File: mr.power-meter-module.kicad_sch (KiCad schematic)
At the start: 3 parts

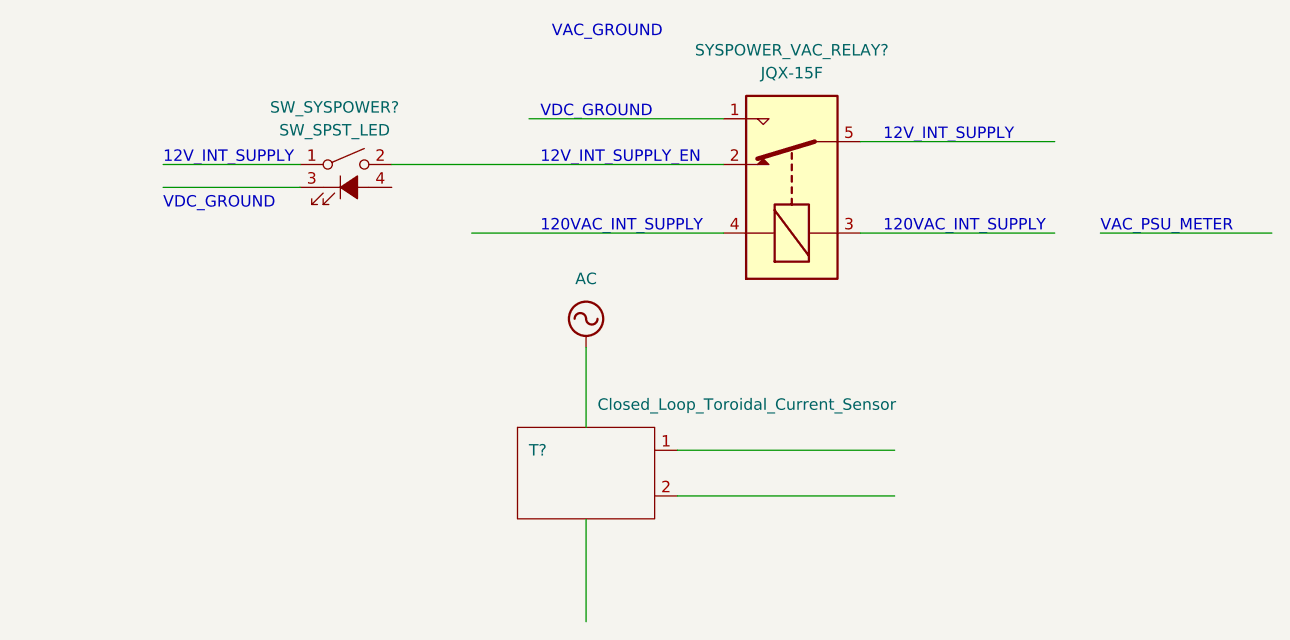
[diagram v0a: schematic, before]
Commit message: Place Holder:
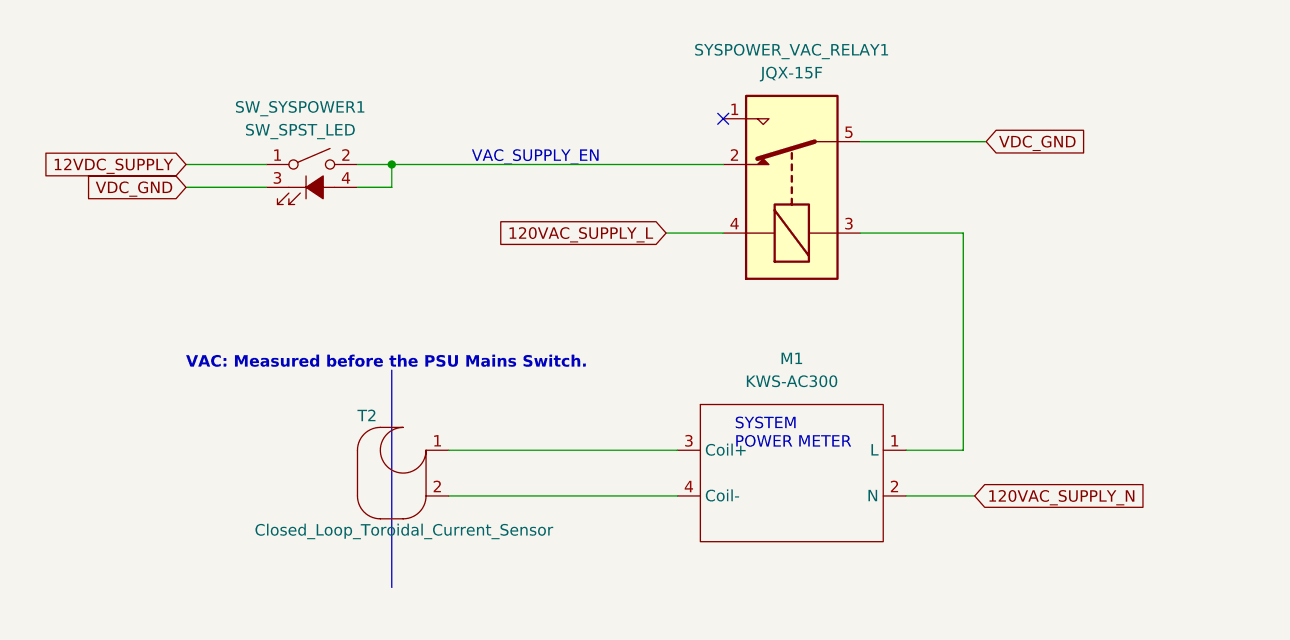
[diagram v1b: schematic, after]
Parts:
- added M1: KWS-AC300, symbol bvm-library:4_Pin_Meter_With_Toroid
- gave numbers to parts that had none: 3
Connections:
- net at SW_SYSPOWER1.2, SYSPOWER_VAC_RELAY1.2: now also SW_SYSPOWER1.4 (A)
- net at SYSPOWER_VAC_RELAY1.3: now also M1.1 (L)
- net 120VAC_SUPPLY_L: now reaches SYSPOWER_VAC_RELAY1.4
- net VDC_GND: now reaches SYSPOWER_VAC_RELAY1.5, SYSPOWER_VAC_RELAY1.6
- net VDC_GND: now also SW_SYSPOWER1.3 (K)
- net at T2.1 (Current_Sense_A): now also M1.3 (Coil+)
- net at T2.2 (Current_Sense_B): now also M1.4 (Coil-)
- net 12VDC_SUPPLY: now reaches SW_SYSPOWER1.1
- new net 120VAC_SUPPLY_N: M1.2 (N)
- no-connect marks 0 -> 1
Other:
- note added: "SYSTEM POWER METER"
- note added: "VAC: Measured before the PSU Mains Switch."
- note added: "VAC_SUPPLY_EN"
- note removed: "120VAC_INT_SUPPLY"
- note removed: "12V_INT_SUPPLY"
- note removed: "12V_INT_SUPPLY_EN"
- note removed: "VAC_GROUND"
- note removed: "VAC_PSU_METER"
- note removed: "VDC_GROUND"
- moved on the sheet: SW_SYSPOWER1
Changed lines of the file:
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@@
     (company "eatmellc")
   )
-  (wire (pts (xy 124.46 63.5) (xy 146.05 63.5))
-    (stroke (width 0) (type default) (color 0 0 0 0))
+  (junction (at 109.22 68.58) (diameter 0) (color 0 0 0 0)
   )
-  (wire (pts (xy 83.82 68.58) (xy 99.06 68.58))
-    (stroke (width 0) (type default) (color 0 0 0 0))
-  )
-  (wire (pts (xy 140.97 100.33) (xy 165.1 100.33))
-    (stroke (width 0) (type default) (color 0 0 0 0))
-  )
-  (wire (pts (xy 187.96 76.2) (xy 207.01 76.2))
-    (stroke (width 0) (type default) (color 0 0 0 0))
-  )
-  (wire (pts (xy 118.11 76.2) (xy 146.05 76.2))
-    (stroke (width 0) (type default) (color 0 0 0 0))
-  )
-  (wire (pts (xy 130.81 107.95) (xy 130.81 119.38))
-    (stroke (width 0) (type default) (color 0 0 0 0))
-  )
-  (wire (pts (xy 83.82 71.12) (xy 99.06 71.12))
+  (no_connect (at 146.05 63.5))
+  (wire (pts (xy 109.22 68.58) (xy 109.22 71.12))
     (stroke (width 0) (type default) (color 0 0 0 0))
   )
@@
     (stroke (width 0) (type default) (color 0 0 0 0))
   )
-  (wire (pts (xy 161.29 66.04) (xy 182.88 66.04))
+  (wire (pts (xy 86.36 68.58) (xy 95.25 68.58))
     (stroke (width 0) (type default) (color 0 0 0 0))
   )
-  (wire (pts (xy 161.29 76.2) (xy 182.88 76.2))
+  (wire (pts (xy 172.72 100.33) (xy 172.72 76.2))
     (stroke (width 0) (type default) (color 0 0 0 0))
   )
-  (wire (pts (xy 140.97 105.41) (xy 165.1 105.41))
+  (wire (pts (xy 109.22 71.12) (xy 105.41 71.12))
     (stroke (width 0) (type default) (color 0 0 0 0))
   )
-  (wire (pts (xy 130.81 88.9) (xy 130.81 97.79))
+  (wire (pts (xy 139.7 76.2) (xy 146.05 76.2))
     (stroke (width 0) (type default) (color 0 0 0 0))
   )
-  (text "12V_INT_SUPPLY" (at 163.83 66.04 0)
+  (wire (pts (xy 166.37 100.33) (xy 172.72 100.33))
+    (stroke (width 0) (type default) (color 0 0 0 0))
+  )
+  (wire (pts (xy 105.41 68.58) (xy 109.22 68.58))
+    (stroke (width 0) (type default) (color 0 0 0 0))
+  )
+  (wire (pts (xy 115.57 100.33) (xy 140.97 100.33))
+    (stroke (width 0) (type default) (color 0 0 0 0))
+  )
+  (wire (pts (xy 161.29 66.04) (xy 175.26 66.04))
+    (stroke (width 0) (type default) (color 0 0 0 0))
+  )
+  (wire (pts (xy 161.29 76.2) (xy 172.72 76.2))
+    (stroke (width 0) (type default) (color 0 0 0 0))
+  )
+  (wire (pts (xy 115.57 105.41) (xy 140.97 105.41))
+    (stroke (width 0) (type default) (color 0 0 0 0))
+  )
+  (polyline (pts (xy 109.22 91.44) (xy 109.22 115.57))
+    (stroke (width 0) (type default) (color 0 0 0 0))
+  )
+  (wire (pts (xy 166.37 105.41) (xy 173.99 105.41))
+    (stroke (width 0) (type default) (color 0 0 0 0))
+  )
+  (wire (pts (xy 86.36 71.12) (xy 95.25 71.12))
+    (stroke (width 0) (type default) (color 0 0 0 0))
+  )
+  (text "VAC_SUPPLY_EN" (at 118.11 68.58 0)
     (effects (font (size 1.27 1.27)) (justify left bottom))
   )
-  (text "VAC_GROUND" (at 127 54.61 0)
+  (text "SYSTEM\nPOWER METER" (at 147.32 100.33 0)
     (effects (font (size 1.27 1.27)) (justify left bottom))
   )
-  (text "VDC_GROUND" (at 83.82 73.66 0)
-    (effects (font (size 1.27 1.27)) (justify left bottom))
+  (text "VAC: Measured before the PSU Mains Switch." (at 86.36 91.44 0)
+    (effects (font (size 1.27 1.27) (thickness 0.254) bold) (justify left bottom))
   )
-  (text "12V_INT_SUPPLY_EN" (at 125.73 68.58 0)
-    (effects (font (size 1.27 1.27)) (justify left bottom))
+  (global_label "120VAC_SUPPLY_L" (shape input) (at 139.7 76.2 180) (fields_autoplaced)
+    (effects (font (size 1.27 1.27)) (justify right))
+    (property "Intersheet References" "${INTERSHEET_REFS}" (id 0) (at 120.0512 76.1206 0)
+      (effects (font (size 1.27 1.27)) (justify right))
+    )
   )
-  (text "VAC_PSU_METER" (at 187.96 76.2 0)
-    (effects (font (size 1.27 1.27)) (justify left bottom))
+  (global_label "VDC_GND" (shape input) (at 175.26 66.04 0)
+    (effects (font (size 1.27 1.27)) (justify left))
+    (property "Intersheet References" "${INTERSHEET_REFS}" (id 0) (at 186.69 66.04 0)
+      (effects (font (size 1.27 1.27)) (justify left))
+    )
   )
-  (text "12V_INT_SUPPLY" (at 83.82 68.58 0)
-    (effects (font (size 1.27 1.27)) (justify left bottom))
+  (global_label "120VAC_SUPPLY_N" (shape input) (at 173.99 105.41 0) (fields_autoplaced)
+    (effects (font (size 1.27 1.27)) (justify left))
+    (property "Intersheet References" "${INTERSHEET_REFS}" (id 0) (at 193.9412 105.3306 0)
+      (effects (font (size 1.27 1.27)) (justify left))
+    )
   )
-  (text "120VAC_INT_SUPPLY" (at 125.73 76.2 0)
-    (effects (font (size 1.27 1.27)) (justify left bottom))
+  (global_label "12VDC_SUPPLY" (shape input) (at 86.36 68.58 180) (fields_autoplaced)
+    (effects (font (size 1.27 1.27)) (justify right))
+    (property "Intersheet References" "${INTERSHEET_REFS}" (id 0) (at 69.735 68.5006 0)
+      (effects (font (size 1.27 1.27)) (justify right))
+    )
   )
-  (text "120VAC_INT_SUPPLY" (at 163.83 76.2 0)
-    (effects (font (size 1.27 1.27)) (justify left bottom))
+  (global_label "VDC_GND" (shape input) (at 86.36 71.12 180) (fields_autoplaced)
+    (effects (font (size 1.27 1.27)) (justify right))
+    (property "Intersheet References" "${INTERSHEET_REFS}" (id 0) (at 75.4802 71.0406 0)
+      (effects (font (size 1.27 1.27)) (justify right))
+    )
   )
-  (text "VDC_GROUND" (at 125.73 63.5 0)
-    (effects (font (size 1.27 1.27)) (justify left bottom))
-  )
-  (symbol (lib_id "power:AC") (at 130.81 88.9 0) (unit 1)
+  (symbol (lib_id "bvm-library:4_Pin_Meter_With_Toroid") (at 148.59 105.41 0) (unit 1)
     (in_bom yes) (on_board yes) (fields_autoplaced)
-    (property "Reference" "#PWR?" (id 0) (at 130.81 91.44 0)
+    (property "Reference" "M1" (id 0) (at 153.67 90.17 0))
+    (property "Value" "KWS-AC300" (id 1) (at 153.67 92.71 0))
+    (property "Footprint" "" (id 2) (at 148.59 105.41 0)
       (effects (font (size 1.27 1.27)) hide)
     )
-    (property "Value" "AC" (id 1) (at 130.81 81.28 0))
-    (property "Footprint" "" (id 2) (at 130.81 88.9 0)
-      (effects (font (size 1.27 1.27)) hide)
-    )
-    (property "Datasheet" "" (id 3) (at 130.81 88.9 0)
+    (property "Datasheet" "" (id 3) (at 148.59 105.41 0)
       (effects (font (size 1.27 1.27)) hide)
     )
     (pin "1")
+    (pin "2")
+    (pin "3")
+    (pin "4")
   )
   (symbol (lib_id "Relay:Y14x-1C-xxDS") (at 153.67 71.12 90) (unit 1)
     (in_bom yes) (on_board yes)
-    (property "Reference" "SYSPOWER_VAC_RELAY?" (id 0) (at 153.67 55.88 90))
+    (property "Reference" "SYSPOWER_VAC_RELAY1" (id 0) (at 153.67 55.88 90))
     (property "Value" "JQX-15F" (id 1) (at 153.67 58.42 90))
     (property "Footprint" "Relay_THT:Relay_SPDT_HsinDa_Y14" (id 2) (at 154.94 59.69 0)
@@
     (pin "6")
   )
-  (symbol (lib_id "bvm-library:Closed_Loop_Toroidal_Current_Sensor") (at 130.81 102.87 0) (unit 1)
+  (symbol (lib_id "bvm-library:Closed_Loop_Toroidal_Current_Sensor") (at 110.49 102.87 0) (unit 1)
     (in_bom yes) (on_board yes)
-    (property "Reference" "T?" (id 0) (at 124.46 100.33 0)
+    (property "Reference" "T2" (id 0) (at 105.41 96.52 0)
       (effects (font (size 1.27 1.27)) (justify left))
     )
-    (property "Value" "Closed_Loop_Toroidal_Current_Sensor" (id 1) (at 132.08 95.25 0)
+    (property "Value" "Closed_Loop_Toroidal_Current_Sensor" (id 1) (at 93.98 109.22 0)
       (effects (font (size 1.27 1.27)) (justify left))
     )
-    (property "Footprint" "" (id 2) (at 130.81 102.87 0)
+    (property "Footprint" "" (id 2) (at 110.49 102.87 0)
       (effects (font (size 1.27 1.27)) hide)
     )
-    (property "Datasheet" "" (id 3) (at 130.81 102.87 0)
+    (property "Datasheet" "" (id 3) (at 110.49 102.87 0)
       (effects (font (size 1.27 1.27)) hide)
     )
@@
     (pin "2")
   )
-  (symbol (lib_id "Switch:SW_SPST_LED") (at 104.14 71.12 0) (unit 1)
+  (symbol (lib_id "Switch:SW_SPST_LED") (at 100.33 71.12 0) (unit 1)
     (in_bom yes) (on_board yes) (fields_autoplaced)
-    (property "Reference" "SW_SYSPOWER?" (id 0) (at 102.87 62.23 0))
-    (property "Value" "SW_SPST_LED" (id 1) (at 102.87 64.77 0))
-    (property "Footprint" "" (id 2) (at 104.14 63.5 0)
+    (property "Reference" "SW_SYSPOWER1" (id 0) (at 99.06 62.23 0))
+    (property "Value" "SW_SPST_LED" (id 1) (at 99.06 64.77 0))
+    (property "Footprint" "" (id 2) (at 100.33 63.5 0)
       (effects (font (size 1.27 1.27)) hide)
     )
-    (property "Datasheet" "~" (id 3) (at 104.14 63.5 0)
+    (property "Datasheet" "~" (id 3) (at 100.33 63.5 0)
       (effects (font (size 1.27 1.27)) hide)
     )
